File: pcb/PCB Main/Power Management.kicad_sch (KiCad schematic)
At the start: 28 parts, among them J1 Conn_01x03, J2 Conn_01x02, J3 Conn_01x02, J4 Conn_01x02, U2 AEM10941, U3 INA3221

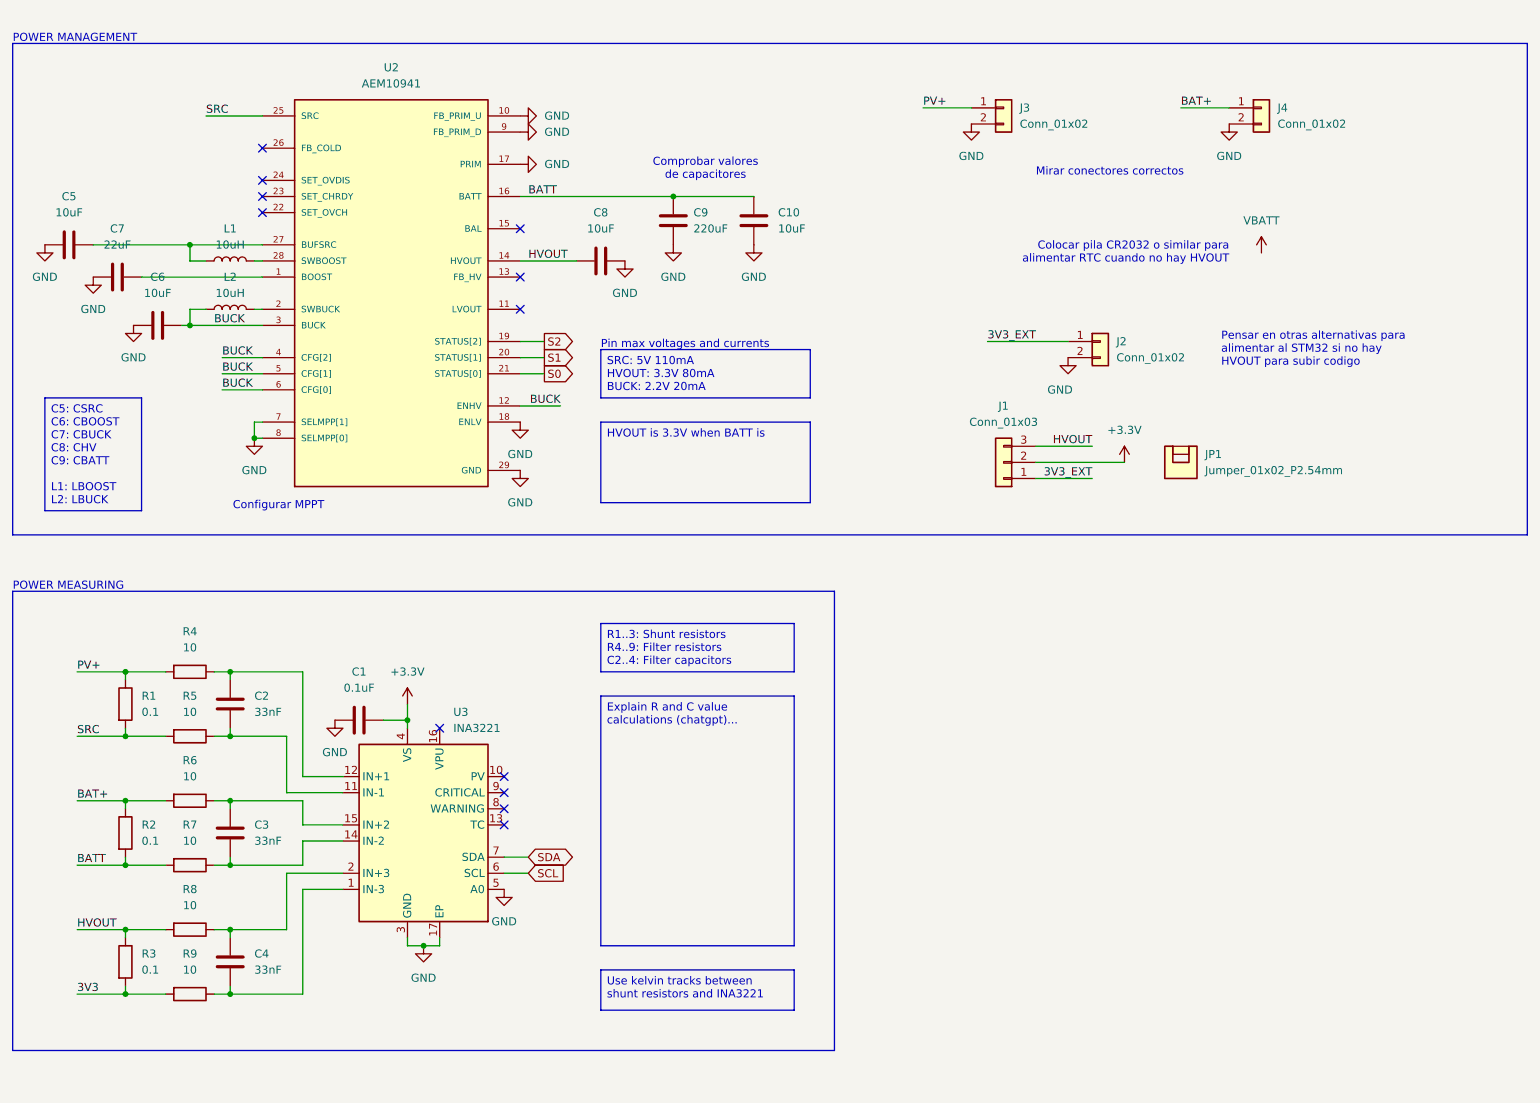
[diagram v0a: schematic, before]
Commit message: PCB casi lista
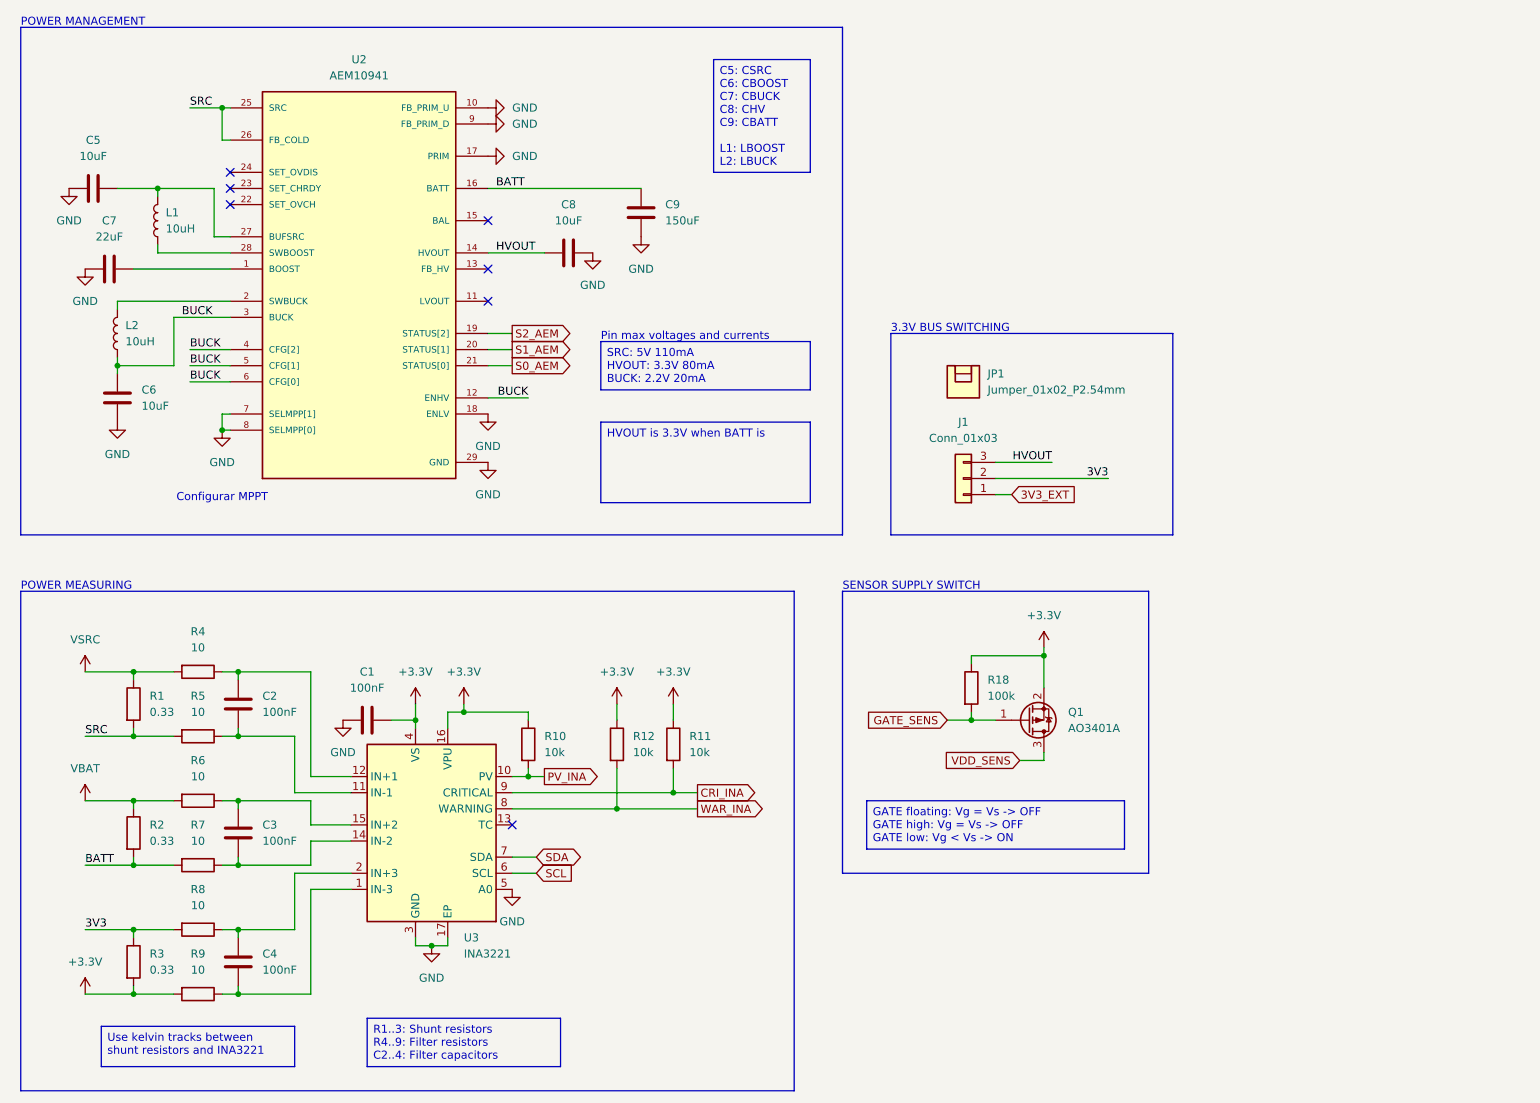
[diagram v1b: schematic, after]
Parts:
- removed C10: 10uF, Capacitor_SMD:C_0805_2012Metric, symbol Device:C
- removed J2: Conn_01x02, Connector_PinHeader_2.54mm:PinHeader_1x02_P2.54mm_Vertical, symbol Connector_Generic:Conn_01x02
- removed J3, J4: Conn_01x02, Connector_PinHeader_1.27mm:PinHeader_1x02_P1.27mm_Vertical, symbol Connector_Generic:Conn_01x02
- added Q1: AO3401A, Package_TO_SOT_SMD:SOT-23, symbol Transistor_FET:AO3401A
- added R10, R11, R12: 10k, Resistor_SMD:R_0402_1005Metric, symbol Device:R
- added R18: 100k, Resistor_SMD:R_0402_1005Metric, symbol Device:R
- C1: value 0.1uF -> 100nF; footprint Capacitor_SMD:C_0603_1608Metric -> Capacitor_SMD:C_0402_1005Metric; Component CC0603KRX7R9BB104 -> CL05B104KO5NNNC; Manufacturer YAGEO -> Samsung; Package C_0603 -> 0402; Supplier Part # C14663 -> C1525; Supplier Part Type (none) -> Basic
- C2, C3, C4: value 33nF -> 100nF; footprint Capacitor_SMD:C_0603_1608Metric -> Capacitor_SMD:C_0402_1005Metric; Component CC0603KRX7R9BB333 -> CL05B104KO5NNNC; Manufacturer YAGEO -> Samsung; Package C_0603 -> 0402; Supplier Part # C106856 -> C1525; Supplier Part Type (none) -> Basic
- C5, C6, C8: footprint Capacitor_SMD:C_0805_2012Metric -> Capacitor_SMD:C_0603_1608Metric; Component GRM21BR71A106KE51L -> CL10A106KP8NNNC; Manufacturer Murata Electronics -> Samsung; Package C_0805 -> 0603; Supplier Part # C86038 -> C19702; Supplier Part Type (none) -> Basic
- C7: footprint Capacitor_SMD:C_0805_2012Metric -> Capacitor_SMD:C_0603_1608Metric; Component GRM21BZ71A226ME15L -> CL10A226MQ8NRNC; Manufacturer Murata Electronics -> Samsung; Package C_0805 -> 0603; Supplier Part # C907991 -> C59461; Supplier Part Type (none) -> Basic
- C9: value 220uF -> 150uF; footprint Capacitor_SMD:CP_Elec_8x6.2 -> Capacitor_SMD:C_1206_3216Metric; Component EEEFK1A221P -> GRM31CR60J157ME11L; Manufacturer PANASONIC -> Murata Electronics; Package SMD (8x6.2) -> 1206; Supplier Part # C401648 -> C528968; Supplier Part Type (none) -> Extended
- J1: Supplier Part Type (none) -> -
- JP1: Supplier Part Type (none) -> Mechanical Assembly
- L1: Package SMD (3.9x3.9) -> SMD 3.9x3.9mm; Supplier Part Type (none) -> Extended
- L2: footprint Inductor_SMD:L_0805_2012Metric -> Inductor_SMD:L_0603_1608Metric; Component MLZ2012N100LT000 -> MLZ1608M100WT000; Package L_0805 -> 0603; Supplier Part # C88182 -> C76798; Supplier Part Type (none) -> Extended
- R1, R2, R3: value 0.1 -> 0.33; Component CSRN2512FTR100 -> RLP25FEER330; Manufacturer SEI(Stackpole Elec) -> TA-I Tech; Package R_2512 -> 2512; Supplier Part # C346817 -> C393076; Supplier Part Type (none) -> Extended
- R4, R5, R6, R7, R8, R9: footprint Resistor_SMD:R_0603_1608Metric -> Resistor_SMD:R_0402_1005Metric; Component RC0603FR-0710RL -> 0402WGF100JTCE; Manufacturer YAGEO -> UNI-ROYAL; Package R_0603 -> 0402; Supplier Part # C109318 -> C25077; Supplier Part Type (none) -> Basic
- U2: Supplier (none) -> Mouser; Supplier Part # (none) -> 120-AEM10941-QFN; Supplier Part Type (none) -> -
- U3: Supplier Part Type (none) -> Extended
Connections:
- net +3.3V: now also R3.2, R9.2, U3.16 (VPU), Q1.2 (S), R10.1, R11.1, R12.1, R18.1; no longer J1.2 (Pin_2)
- net 3V3: now also J1.2 (Pin_2), R3.1, R8.2; no longer R3.2, R9.2
- net BATT: now also C9.1; no longer C9.2
- net GND: now also C9.2; no longer C9.1
- net HVOUT: no longer R3.1, R8.2
- net SRC: now also U2.26 (FB_COLD)
- net PV_INA: now reaches U3.10 (PV)
- net PV_INA: now also R10.2
- net WAR_INA: now reaches U3.8 (WARNING)
- net WAR_INA: now also R12.2
- net CRI_INA: now reaches U3.9 (CRITICAL)
- net CRI_INA: now also R11.2
- net at C5.1, U2.27 (BUFSRC): now also L1.2; no longer L1.1
- net at U2.28 (SWBOOST): now also L1.1; no longer L1.2
- net BAT+ renamed VBAT
- net PV+ renamed VSRC
- net S0 renamed S0_AEM
- net S1 renamed S1_AEM
- net S2 renamed S2_AEM
- new net GATE_SENS: Q1.1 (G), R18.2
- new net VDD_SENS: Q1.3 (D)
- no-connect marks 12 -> 7
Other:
- note added: "3.3V BUS SWITCHING"
- note added: "SENSOR SUPPLY SWITCH"
- note removed: "Colocar pila CR2032 o similar para alimentar RTC cuando no hay HVOUT"
- note removed: "Comprobar valores de capacitores"
- note removed: "Mirar conectores correctos"
- note removed: "Pensar en otras alternativas para alimentar al STM32 si no hay HVOUT para subir codigo"
- moved on the sheet: C1, C2, C3, C4, C5, C6, C7, C8, J1, JP1, L1, L2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
